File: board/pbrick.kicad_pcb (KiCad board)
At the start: 4 copper layers, 24 x 44 mm, 58 parts, among them J1 UJC-HP-3-SMT-TR, J2 TC2030-IDC-NL, J3 U.FL2PIN, J4 QWIIC, M0 5055680471, M1 5055680471, Q1 SSM6J507NU, Q2 SSM6J507NU, U1 MIC5219-3.3YML-TR, U2 ADP3330ARTZ-5-RL7, U3 STUSB4500QTR, U5 TB67H420FTG(O,EL), U6 2533020201601, U7 PCA9624

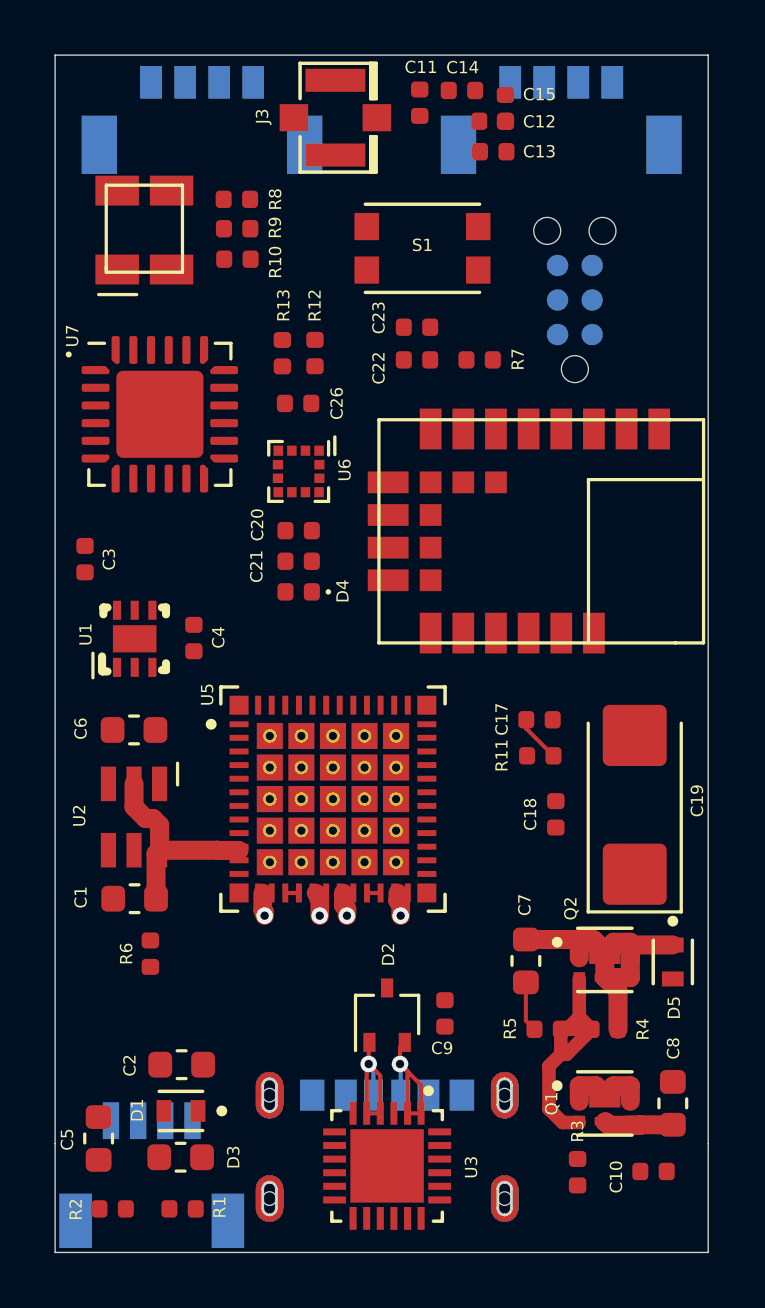
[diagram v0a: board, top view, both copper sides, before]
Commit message: Updating PCB routing
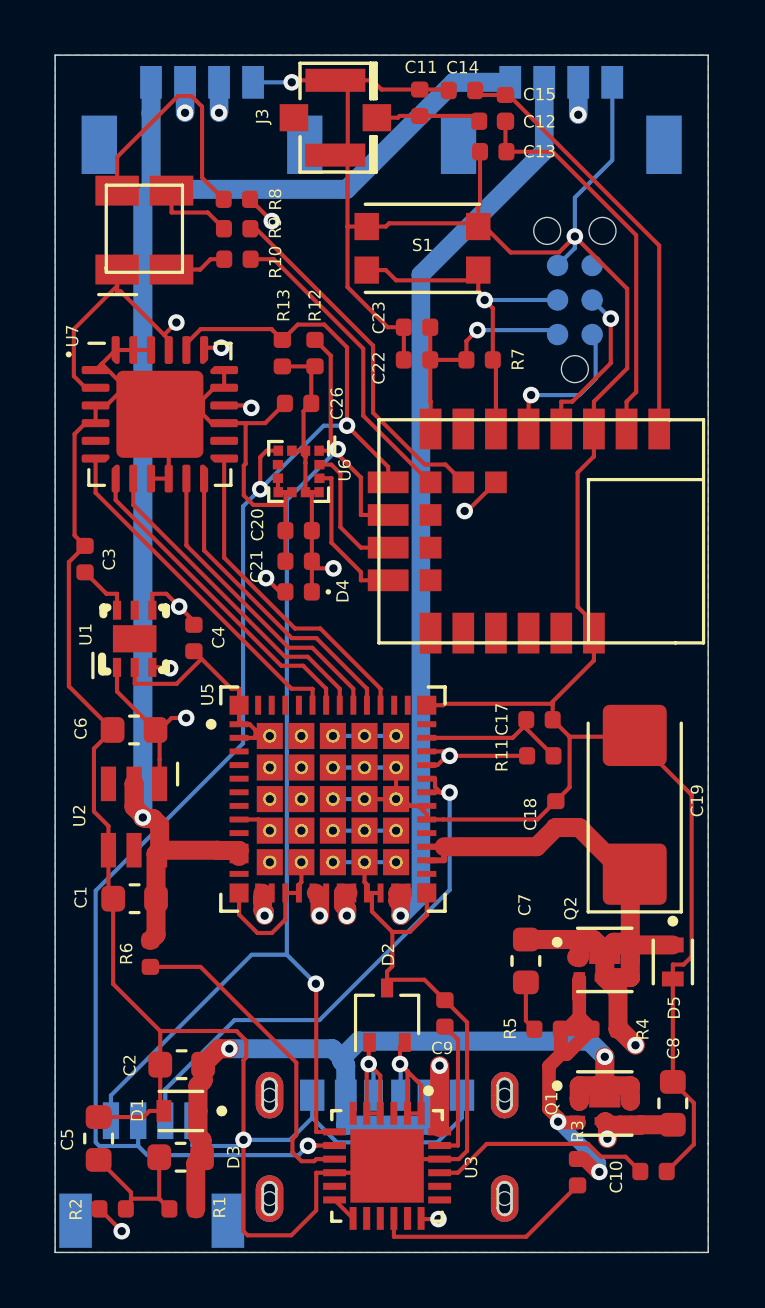
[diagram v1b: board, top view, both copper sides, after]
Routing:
- net GND: track 1.00 -> 303.0 mm, vias 0 -> 3
- net VDD: track 24.4 -> 112.5 mm, vias 0 -> 4
- net 3.3V: track 0.00 -> 63.0 mm, vias 0 -> 3
- net /P0.19: track 0.00 -> 55.3 mm, vias 0 -> 3
- net /P0.22: track 0.00 -> 51.8 mm, vias 0 -> 3
- net 5V: track 0.00 -> 49.8 mm, vias 0 -> 5
- net /M1_0: track 0.89 -> 36.3 mm, vias 1 -> 2
- net /M0_0: track 0.89 -> 36.1 mm, vias 1 -> 2
- net /M1_1: track 0.86 -> 35.4 mm, vias 1 -> 2
- net /M0_1: track 0.88 -> 34.2 mm
- net VBUS: track 3.29 -> 32.9 mm, vias 0 -> 2
- net /P0.09: track 0.00 -> 16.3 mm, vias 0 -> 2
- net /ANT: track 0.00 -> 15.9 mm
- net /RF: track 0.00 -> 14.4 mm
- net Net-(R2-Pad2): track 0.00 -> 13.8 mm, vias 0 -> 2
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- added copper zone on B.Cu, net GND
- added copper zone on GND, net GND
- added copper zone on M.Cu, net GND
- added copper zone on M.Cu, net VBUS
- added copper zone on M.Cu, net VDD
